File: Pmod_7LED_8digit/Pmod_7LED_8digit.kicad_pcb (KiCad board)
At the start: 2 copper layers, 99.6 x 20.3 mm, 16 parts, among them J1 Pmod_Header, U1 74HC595, U2 74HC595

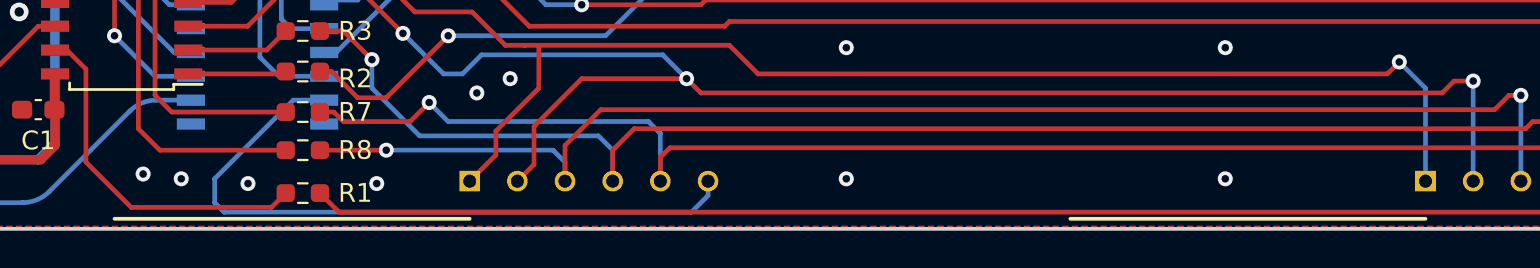
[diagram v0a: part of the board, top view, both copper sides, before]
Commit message: 0811
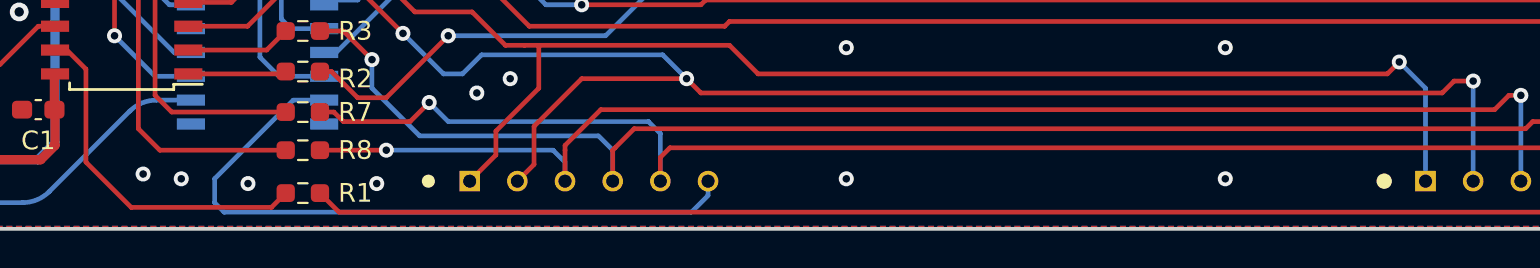
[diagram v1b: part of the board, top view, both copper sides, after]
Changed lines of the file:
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@@
         (effects (font (size 1.27 1.27) (thickness 0.254)))
     )
-    (fp_line (start -2.005 -18.925) (end -2.005 0)
-      (stroke (width 0.2) (type solid)) (layer "F.SilkS"))
+    (fp_circle (center 0 -2.2) (end 0.3 -2.2)
+      (stroke (width 0.1) (type solid)) (fill solid) (layer "F.SilkS"))
     (fp_line (start -2.255 -19.175) (end 17.495 -19.175)
       (stroke (width 0.05) (type solid)) (layer "F.CrtYd"))
@@
         (effects (font (size 1.27 1.27) (thickness 0.254)))
     )
-    (fp_line (start -2.005 -18.925) (end -2.005 0)
-      (stroke (width 0.2) (type solid)) (layer "F.SilkS"))
+    (fp_circle (center 0 -2.2) (end 0.360555 -2.2)
+      (stroke (width 0.1) (type solid)) (fill solid) (layer "F.SilkS"))
     (fp_line (start -2.255 -19.175) (end 17.495 -19.175)
       (stroke (width 0.05) (type solid)) (layer "F.CrtYd"))
